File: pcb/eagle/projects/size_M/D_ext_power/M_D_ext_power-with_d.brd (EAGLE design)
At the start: 34 parts

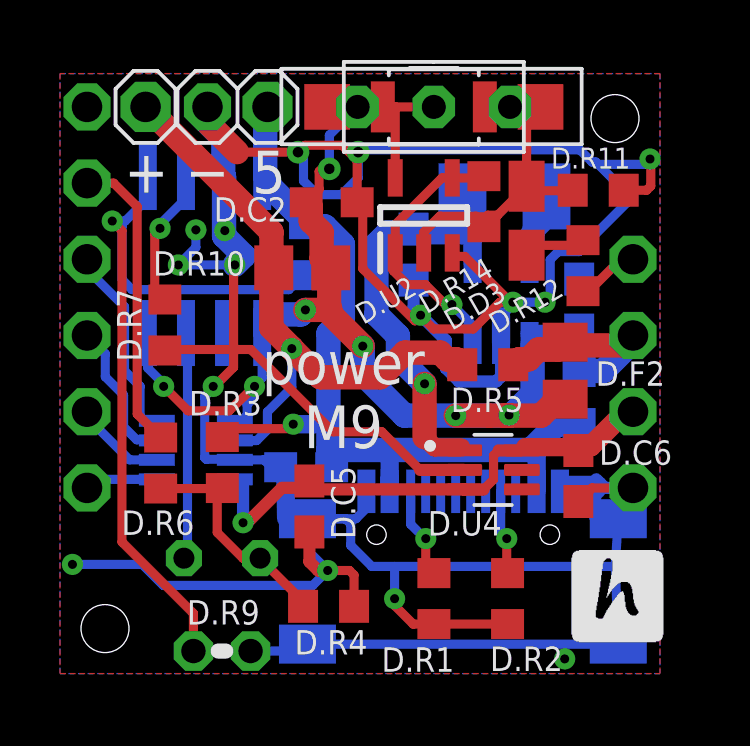
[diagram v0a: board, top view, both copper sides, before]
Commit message: just renamed
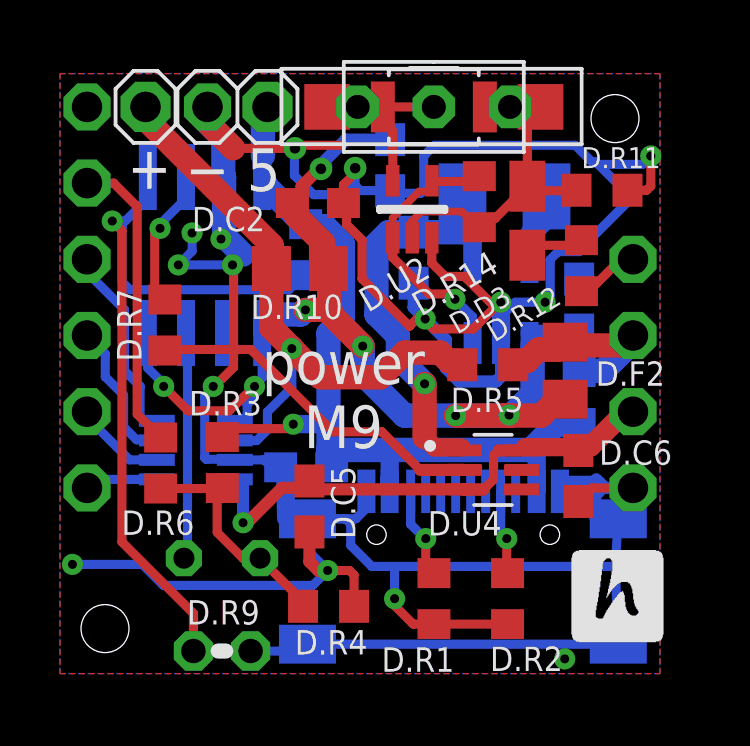
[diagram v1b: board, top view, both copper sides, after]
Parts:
- added D.C7: 100n, rcl:C0603
- D.U2: value 74LVC1G80GV,125 -> SN74AUP1G80; device 74LVC1G80GV_125:SOT95P275X110-5N -> SN74AUP1G80DCKR:DCK0005A_M
- moved D.C2 0.46 mm to (9.10, 16.2)
- moved D.U2 0.43 mm to (12.2, 16.0)
- moved D.R14 0.15 mm to (14.5, 16.2), turned to 90 degrees
- moved D.R11 0.13 mm to (18.6, 16.6)
- moved D.C4 0.10 mm to (12.3, 14.4)
- moved D.R10 0.08 mm to (8.50, 14.0)
- moved D.R12 0.05 mm to (17.9, 14.1)
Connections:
- removed net N$1: D.R14.1, D.U2.1, D.U2.4, D.U3.SHDN
- new net N$9: D.R14.2, D.U2.1, D.U2.4, D.U3.SHDN
- net GND: now also D.C7.1
- net IN+: now also D.C7.2
- net N$10: now also D.R14.1; no longer D.R14.2
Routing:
- net N$9: track 0.00 -> 9.53 mm, vias 0 -> 1
- net N$1: track 9.17 -> 0.00 mm, vias 1 -> 0
- net IN+: track 45.4 -> 48.1 mm
- net GND: track 145.4 -> 146.9 mm
- net N$10: track 13.4 -> 14.0 mm
